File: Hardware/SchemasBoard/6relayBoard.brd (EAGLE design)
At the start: 53.1 x 41.8 mm, 46 parts, among them IC1 LNK304, IC3 MC33269ST-3.3T3, K1 FRS1B, K2 FRS1B, K3 FRS1B, K4 FRS1B, K5 FRS1B, K6 FRS1B, T1 BC846, T2 BC846, T3 BC846, T4 BC846, T5 BC846, T6 BC846

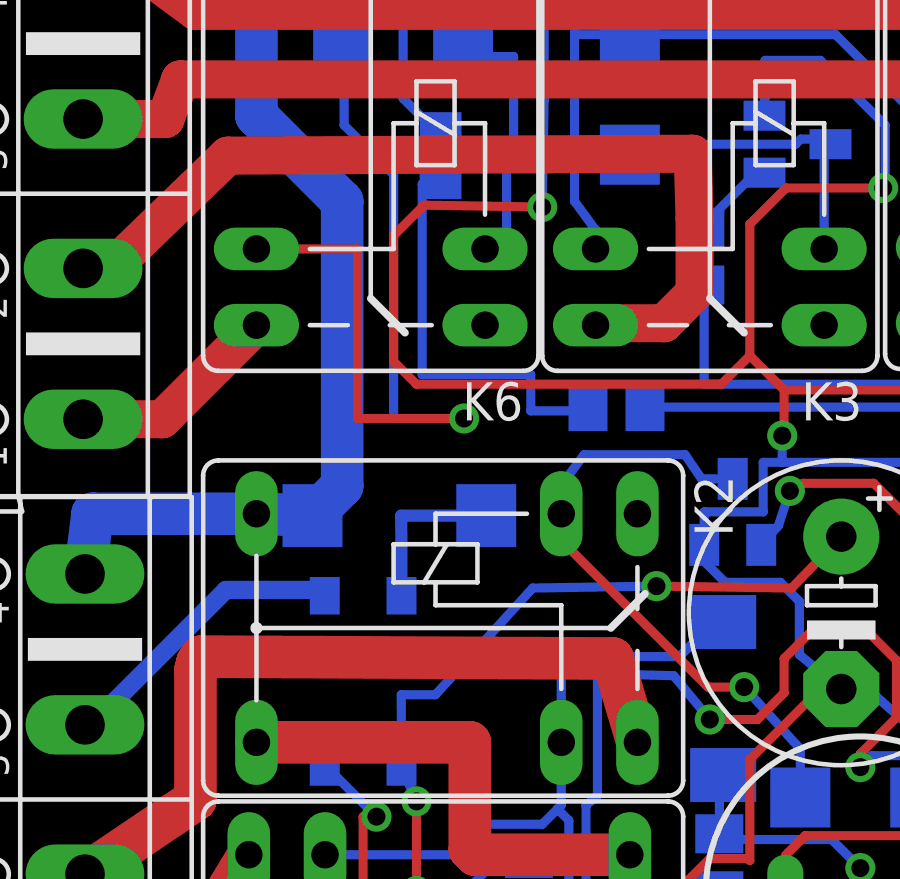
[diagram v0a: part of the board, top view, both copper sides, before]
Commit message: asd
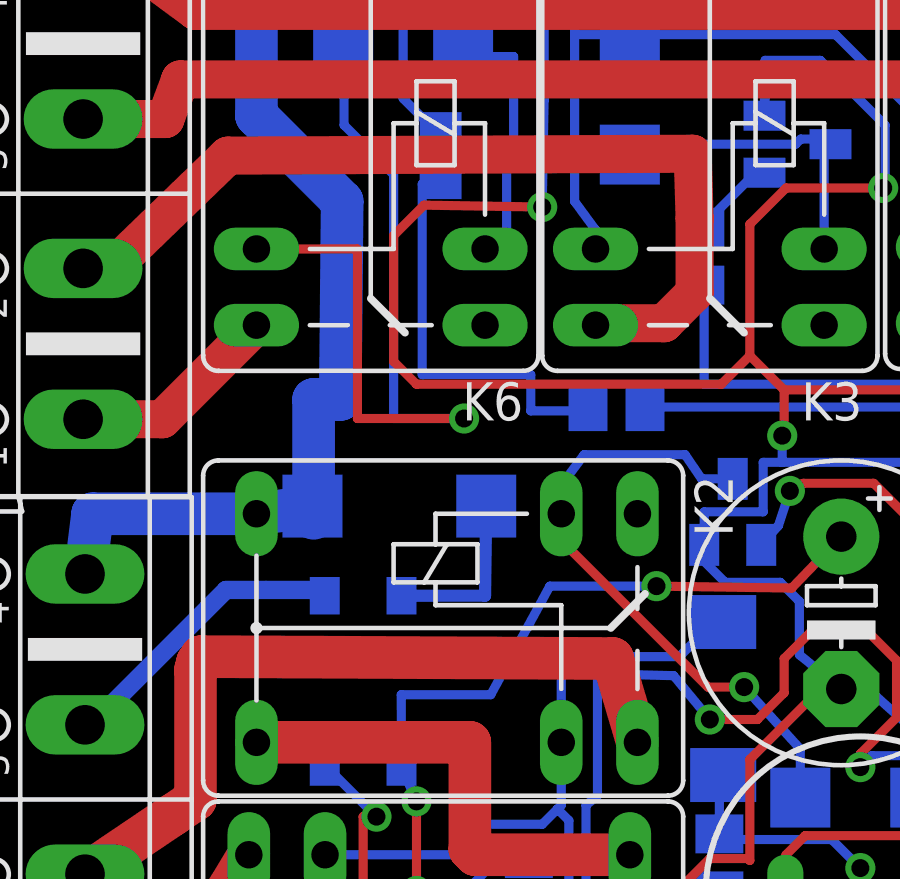
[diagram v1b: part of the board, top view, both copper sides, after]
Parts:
- moved R2 0.32 mm to (13.1, 21.1)
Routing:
- net N$36: track 79.5 -> 80.3 mm
- net N$2: track 30.8 -> 31.4 mm
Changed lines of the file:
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@@
 <element name="B1" library="rectifier" package="TO-269AA" value="RECTIFIER" x="11.938" y="15.3035" rot="MR0"/>
 <element name="R1" library="resistor" package="R2512W" value="100" x="9.906" y="5.715" rot="MR180"/>
-<element name="R2" library="resistor" package="R2512W" value="8,2" x="13.1445" y="20.828" rot="MR180"/>
+<element name="R2" library="resistor" package="R2512W" value="8,2" x="13.1445" y="21.1455" rot="MR180"/>
 <element name="U$1" library="rfm70" package="RFM70" value="RFM70" x="48.5775" y="1.2065" rot="R180"/>
 <element name="U$2" library="microchip" package="SSOP20" value="PIC16F690" x="43.6245" y="11.6205" rot="MR90"/>
@@
 <wire x1="13.716" y1="8.3185" x2="12.192" y2="7.747" width="0.3048" layer="16"/>
 <wire x1="12.192" y1="7.747" x2="7.01" y2="5.715" width="0.3048" layer="16"/>
-<wire x1="13.208" y1="14.859" x2="14.351" y2="14.859" width="0.3048" layer="16"/>
-<wire x1="14.351" y1="14.859" x2="17.5895" y2="18.415" width="0.3048" layer="16"/>
-<wire x1="17.5895" y1="18.415" x2="21.717" y2="18.4785" width="0.3048" layer="16"/>
+<wire x1="13.208" y1="14.859" x2="16.1925" y2="14.859" width="0.3048" layer="16"/>
+<wire x1="16.1925" y1="14.859" x2="18.161" y2="18.4785" width="0.3048" layer="16"/>
+<wire x1="18.161" y1="18.4785" x2="21.717" y2="18.4785" width="0.3048" layer="16"/>
 <via x="21.717" y="18.4785" extent="1-16" drill="0.6"/>
 <wire x1="21.717" y1="18.4785" x2="26.2255" y2="18.415" width="0.3048" layer="1"/>
@@
 <contactref element="R2" pad="2"/>
 <contactref element="B1" pad="AC1"/>
-<wire x1="13.218" y1="18.1585" x2="13.208" y2="20.828" width="0.4064" layer="16"/>
-<wire x1="13.208" y1="20.828" x2="16.0405" y2="20.828" width="0.4064" layer="16"/>
+<wire x1="13.218" y1="18.1585" x2="16.002" y2="18.161" width="0.4064" layer="16"/>
+<wire x1="16.002" y1="18.161" x2="16.0405" y2="21.1455" width="0.4064" layer="16"/>
 </signal>
 <signal name="N$4">
@@
 <wire x1="8.382" y1="39.878" x2="8.382" y2="34.163" width="1.4224" layer="16"/>
 <wire x1="8.382" y1="34.163" x2="11.2395" y2="31.3055" width="1.4224" layer="16"/>
-<wire x1="11.2395" y1="31.3055" x2="11.2395" y2="21.819" width="1.4224" layer="16"/>
-<wire x1="11.2395" y1="21.819" x2="10.2485" y2="20.828" width="1.4224" layer="16"/>
-<wire x1="10.2485" y1="20.828" x2="8.509" y2="20.8915" width="1.4224" layer="16"/>
+<wire x1="11.2395" y1="31.3055" x2="11.176" y2="24.7015" width="1.4224" layer="16"/>
+<wire x1="11.176" y1="24.7015" x2="10.287" y2="24.7015" width="1.4224" layer="16"/>
+<wire x1="10.287" y1="24.7015" x2="10.287" y2="20.93" width="1.4224" layer="16"/>
+<wire x1="10.287" y1="20.7395" x2="10.287" y2="20.93" width="1.4224" layer="16"/>
+<wire x1="10.287" y1="20.93" x2="10.2485" y2="21.1455" width="1.4224" layer="16"/>
+<wire x1="10.2485" y1="21.1455" x2="8.509" y2="20.8915" width="1.4224" layer="16"/>
 <wire x1="8.509" y1="20.8915" x2="8.382" y2="20.8915" width="1.27" layer="16"/>
 </signal>
